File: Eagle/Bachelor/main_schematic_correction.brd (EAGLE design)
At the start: 63 x 76 mm, 112 parts, among them Q2 16MHz, SW7 SPST_TACT-EVQQ2, SW8 SPST_TACT-EVQQ2, SW9 SPST_TACT-EVQQ2, U1 ATMEGA32U4-AU, U2 ADP2302ARDZ-5.0-R7, X1 MICROMATCH-4, X2 MICROMATCH-4, X3 MICROMATCH-4

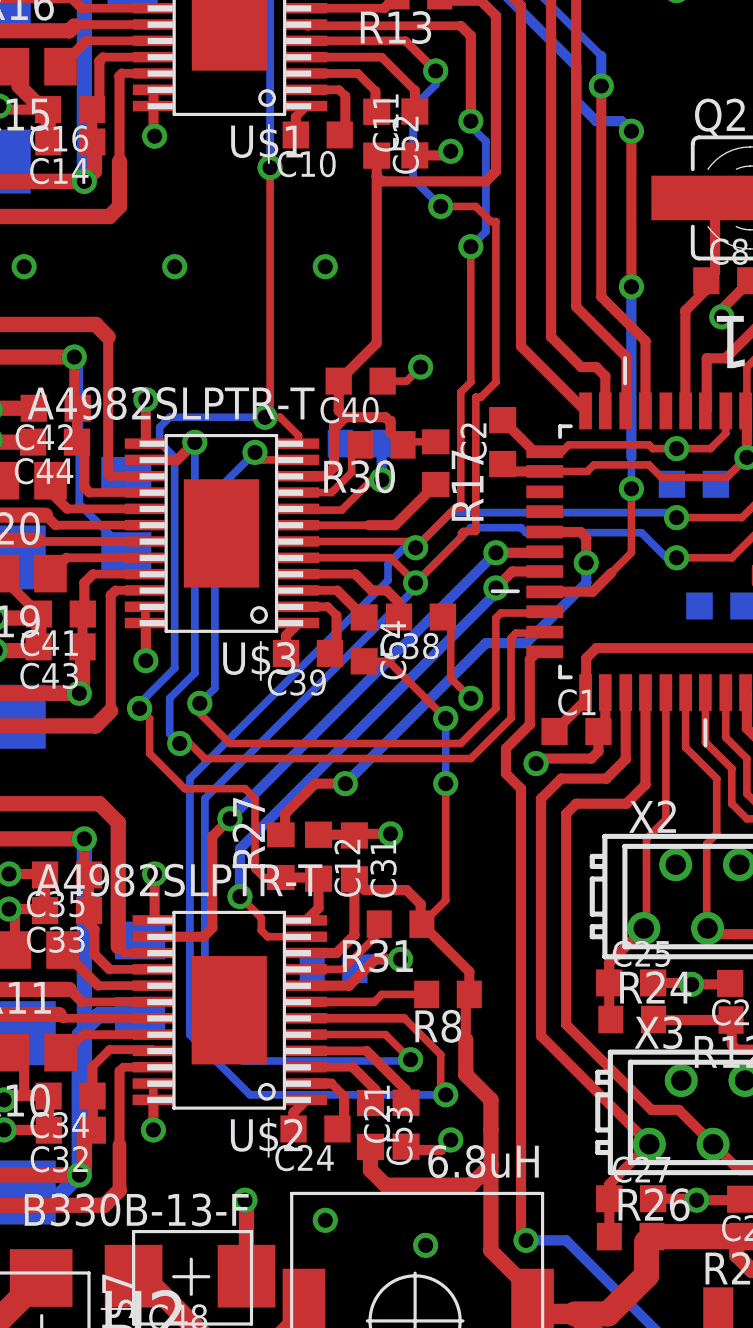
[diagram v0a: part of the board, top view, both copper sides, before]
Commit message: Done
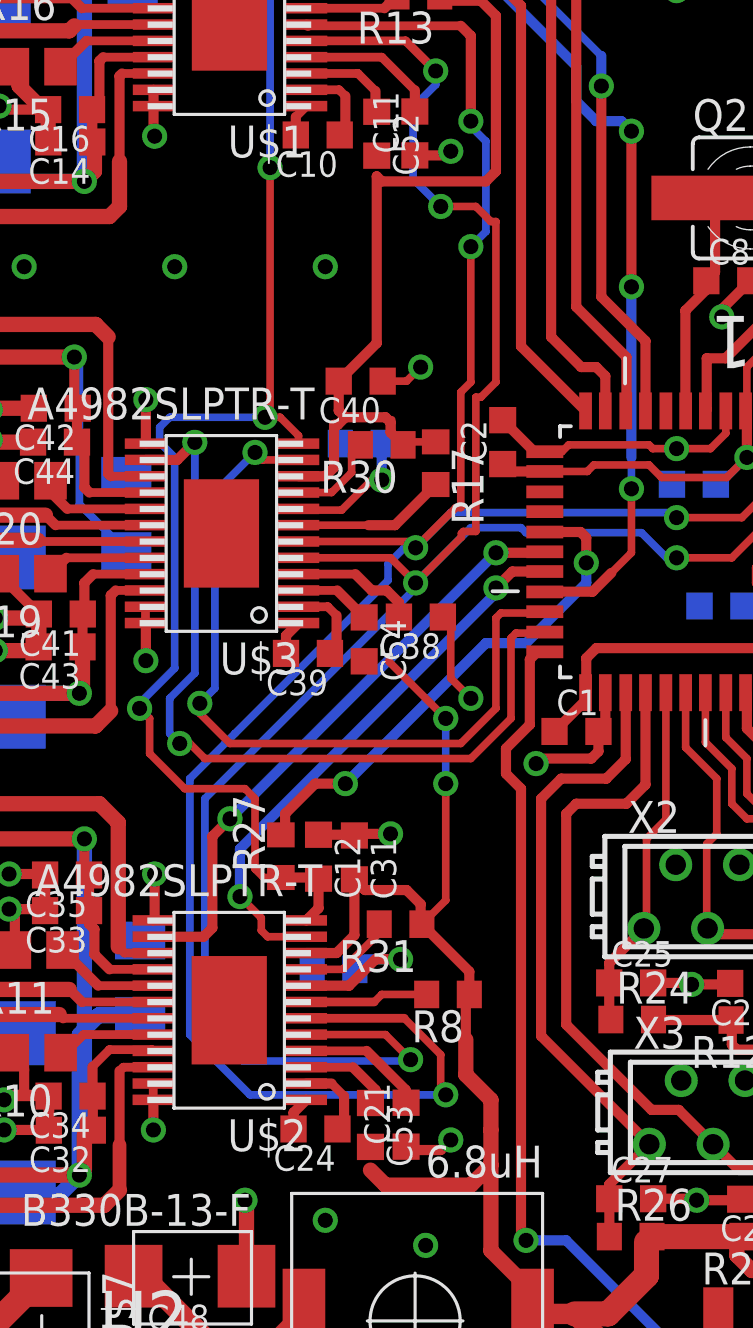
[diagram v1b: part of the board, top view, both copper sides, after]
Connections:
- new net N$134: C52.2
- new net N$135: C53.2
- new net N$136: C54.2
- net VCC: no longer C52.2, C53.2, C54.2
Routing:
- net VCC: track 386.4 -> 383.7 mm
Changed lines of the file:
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@@
 <contactref element="C40" pad="2"/>
 <contactref element="U$3" pad="P10"/>
-<contactref element="C52" pad="2"/>
-<contactref element="C53" pad="2"/>
-<contactref element="C54" pad="2"/>
 <contactref element="U$6" pad="P$1"/>
 <contactref element="C49" pad="2"/>
@@
 <wire x1="45.9734" y1="43.4274" x2="48.1974" y2="43.4274" width="0.4064" layer="1"/>
 <wire x1="48.1974" y1="43.4274" x2="48.7" y2="43.93" width="0.4064" layer="1"/>
-<wire x1="27.8" y1="18.925" x2="27.8" y2="18" width="0.6096" layer="1"/>
 <wire x1="27.8" y1="18" x2="28.4" y2="17.4" width="0.6096" layer="1"/>
 <wire x1="28.4" y1="17.4" x2="31.8" y2="17.4" width="0.6096" layer="1"/>
@@
 <wire x1="36.7" y1="46.1" x2="38.9" y2="46.1" width="0.3048" layer="1"/>
 <wire x1="42" y1="45.6" x2="42.8" y2="46.4" width="0.3048" layer="1"/>
-<wire x1="27.55" y1="38.275" x2="28.525" y2="38.275" width="0.3048" layer="1"/>
 <wire x1="28.525" y1="38.275" x2="30.8" y2="36" width="0.3048" layer="1"/>
 <via x="30.8" y="36" extent="1-16" drill="0.6"/>
@@
 <wire x1="28.05" y1="57.6" x2="28.05" y2="50.955" width="0.4064" layer="1"/>
 <wire x1="28.05" y1="50.955" x2="26.535" y2="49.44" width="0.4064" layer="1"/>
-<wire x1="28.05" y1="57.6" x2="28.05" y2="58.425" width="0.4064" layer="1"/>
 <wire x1="42" y1="45.6" x2="39.4" y2="45.6" width="0.3048" layer="1"/>
 <wire x1="36.7" y1="46.1" x2="36.4404" y2="45.8404" width="0.3048" layer="1"/>
@@
 <via x="60" y="66" extent="1-16" drill="0.6"/>
 </signal>
+<signal name="N$134">
+<contactref element="C52" pad="2"/>
+</signal>
+<signal name="N$135">
+<contactref element="C53" pad="2"/>
+</signal>
+<signal name="N$136">
+<contactref element="C54" pad="2"/>
+</signal>
 </signals>
